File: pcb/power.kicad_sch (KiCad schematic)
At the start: 21 parts, among them IC3 XC6227C331MR-G, IC6 BQ24073RGTR, U3 CR2032-BS-6-1

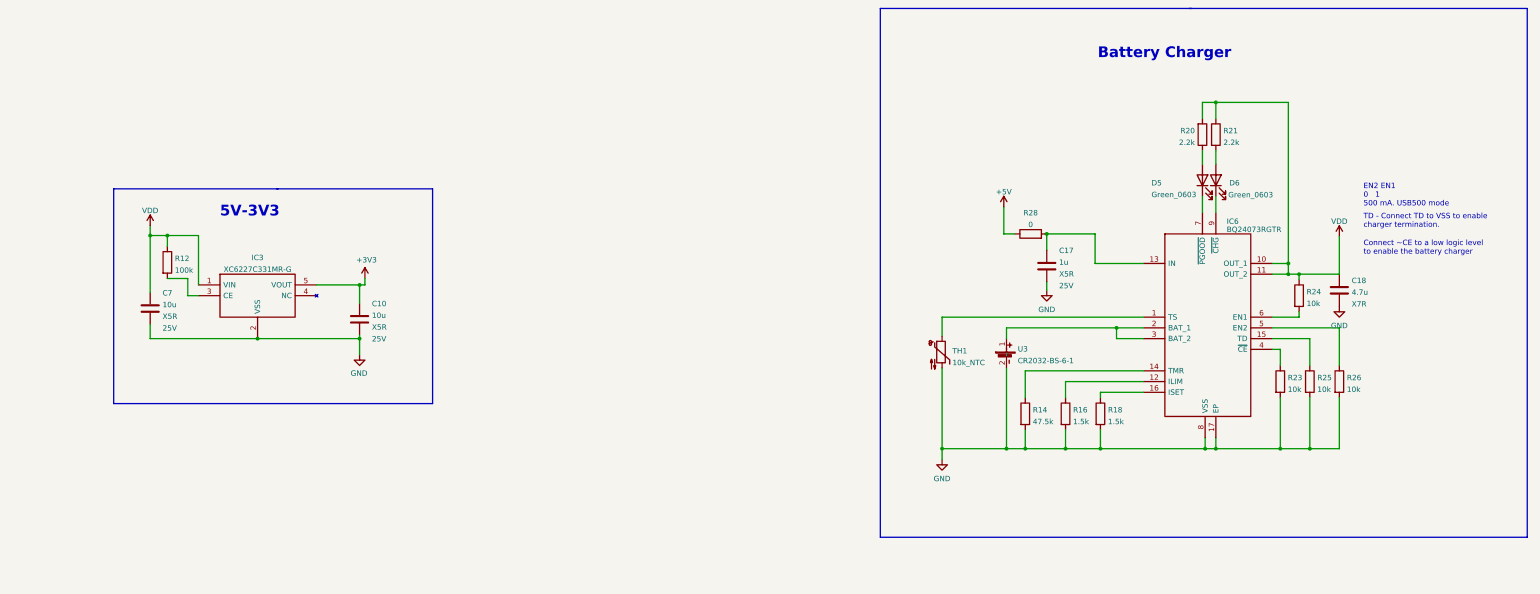
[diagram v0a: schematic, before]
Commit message: Completed initial schematic
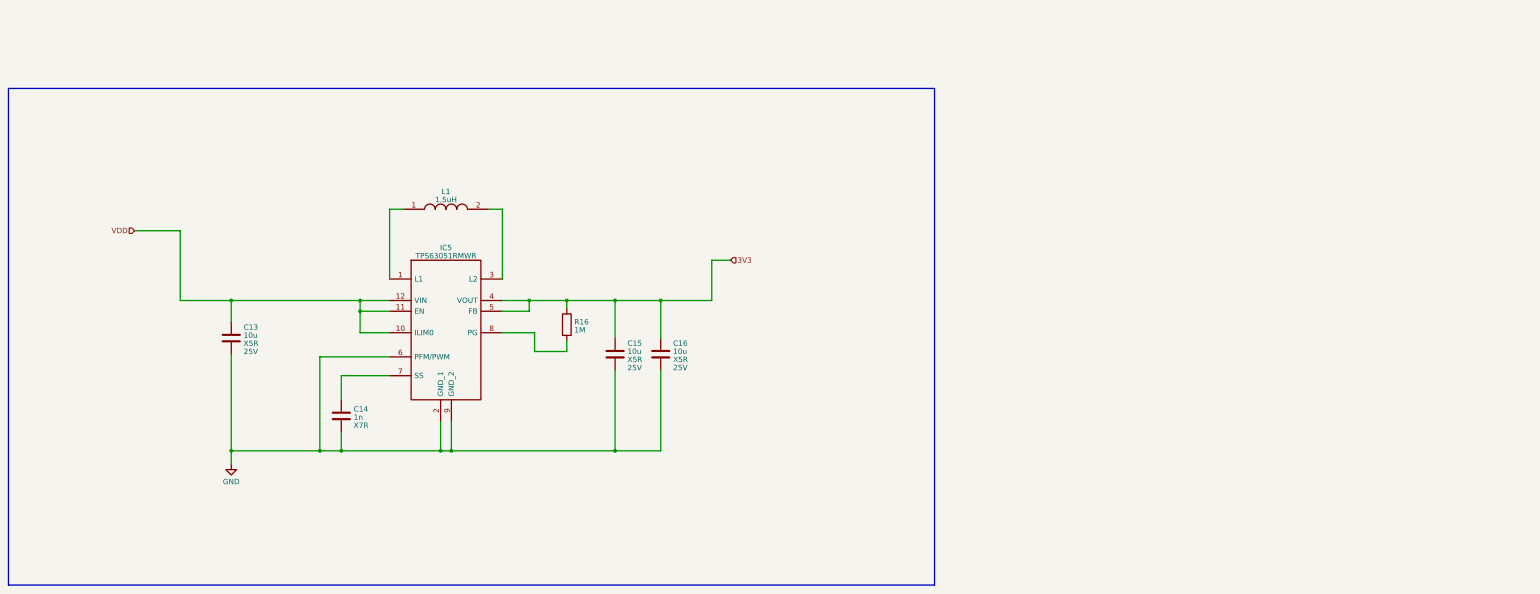
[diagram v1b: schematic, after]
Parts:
- removed C10, C7: 10u, Capacitor_SMD:C_0805_2012Metric, symbol Capacitor_JLC:10u
- removed C17: 1u, Capacitor_SMD:C_0402_1005Metric, symbol Capacitor_JLC:1u
- removed C18: 4.7u, Capacitor_SMD:C_1206_3216Metric, symbol Capacitor_JLC:4.7u
- removed D5, D6: Green_0603, LED_SMD:LED_0603_1608Metric, symbol Diode_JLC:Green_0603
- removed IC3: XC6227C331MR-G, SOT95P280X130-5N, symbol Power-Drivers_JLC:XC6227C331MR-G
- removed IC6: BQ24073RGTR, QFN50P300X300X100-17N-D, symbol Power-Drivers_JLC:BQ24073RGTR
- removed R12: 100k, Resistor_SMD:R_0402_1005Metric, symbol Resistor_JLC:100k
- removed R14: 47.5k, Resistor_SMD:R_0402_1005Metric, symbol Resistor_JLC:47.5k
- removed R16, R18: 1.5k, Resistor_SMD:R_0402_1005Metric, symbol Resistor_JLC:1.5k
- removed R20, R21: 2.2k, Resistor_SMD:R_0402_1005Metric, symbol Resistor_JLC:2.2k
- removed R23, R24, R25, R26: 10k, Resistor_SMD:R_0402_1005Metric, symbol Resistor_JLC:10k
- removed R28: 0, Resistor_SMD:R_0805_2012Metric_Pad1.20x1.40mm_HandSolder, symbol Resistor_JLC:0
- removed TH1: 10k_NTC, Resistor_SMD:R_0402_1005Metric, symbol Resistor_JLC:10k_NTC
- removed U3: CR2032-BS-6-1, CR2032BS61, symbol BatteryHolder_JLC:CR2032-BS-6-1
- added C13, C15, C16: 10u, Capacitor_SMD:C_0805_2012Metric, symbol Capacitor_JLC:10u
- added C14: 1n, Capacitor_SMD:C_0402_1005Metric, symbol Capacitor_JLC:1n
- added IC5: TPS63051RMWR, QFN50P250X250X100-12N-D, symbol Power-Drivers_JLC:TPS63051RMWR
- added L1: 1.5uH, Inductor_SMD:L_0805_2012Metric, symbol Inductor_JLC:1.5uH
- added R16: 1M, Resistor_SMD:R_0402_1005Metric, symbol Resistor_JLC:1M
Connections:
- net GND: now also C13.2, C14.2, C15.2, C16.2, IC5.2 (GND_1), IC5.6 (PFM/PWM), IC5.9 (GND_2)
- net VDD: now also C13.1, IC5.10 (ILIM0), IC5.11 (EN), IC5.12 (VIN)
- new net: IC5.1 (L1), L1.1
- new net: IC5.3 (L2), L1.2
- new net: C14.1, IC5.7 (SS)
- new net: IC5.8 (PG), R16.2
- new net 3V3: C15.1, C16.1, IC5.4 (VOUT), IC5.5 (FB), R16.1
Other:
- note removed: "5V-3V3"
- note removed: "Battery Charger"
- note removed: "Connect ~CE to a low logic level to enable the battery charger"
- note removed: "EN2 EN1 0 1 500 mA. USB500 mode"
- note removed: "TD - Connect TD to VSS to enable charger termination."
